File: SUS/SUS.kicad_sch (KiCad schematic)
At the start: 67 parts, among them J1 ESP32_Connector_0, J2 ESP32_Connector_1, J3 I2C, J4 I2C, J5 I2C, J6 ADC, J7 WS, U1 TJA1051T, U2 ADS8320EB_250, U3 ICM-42688-P, U4 S1001-46R, U5 S1001-46R, U6 S1001-46R

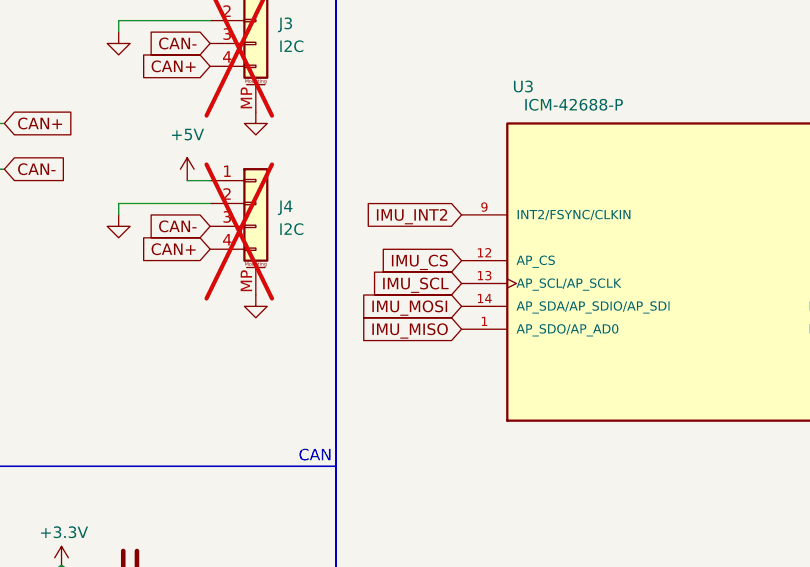
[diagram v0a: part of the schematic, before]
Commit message: Removed Vias
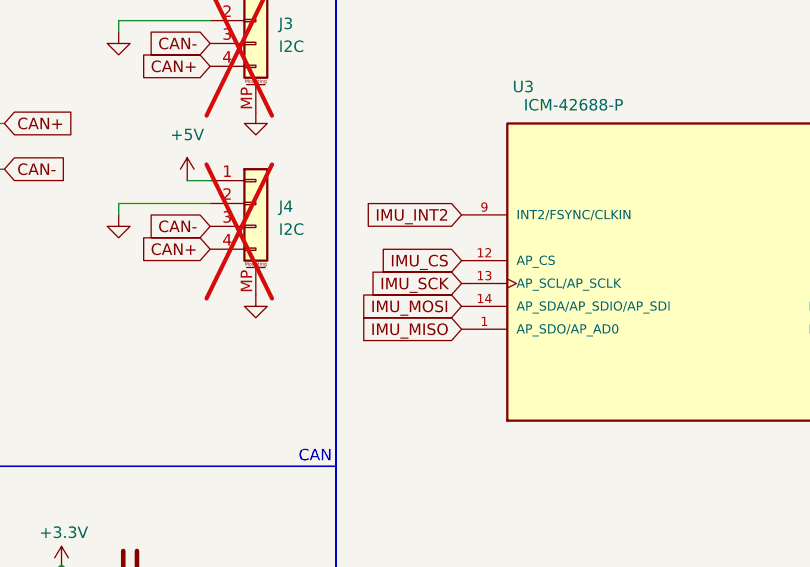
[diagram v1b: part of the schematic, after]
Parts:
- U3: footprint ICM-42688-P:PQFN50P300X250X97-14N -> IMU:ICM-42688-P
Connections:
- net IMU_SCL is gone; now on net IMU_SCK: U3.13 (AP_SCL/AP_SCLK)
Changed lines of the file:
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@@
 		)
 	)
-	(global_label "IMU_SCL"
+	(global_label "IMU_SCK"
 		(shape input)
 		(at 118.11 52.07 180)
@@
 		)
 		(property "Intersheetrefs" "${INTERSHEET_REFS}"
-			(at 107.2629 52.07 0)
+			(at 107.021 52.07 0)
 			(effects
 				(font
@@
 			)
 		)
-		(property "Footprint" "ICM-42688-P:PQFN50P300X250X97-14N"
+		(property "Footprint" "IMU:ICM-42688-P"
 			(at 143.51 49.53 0)
 			(effects
